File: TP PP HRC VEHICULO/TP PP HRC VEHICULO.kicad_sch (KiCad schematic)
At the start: 56 parts, among them J10 Conn_01x04_Pin, J2 Conn_01x01_Pin, J3 Conn_01x01_Pin, J5vgnd1 Screw_Terminal_01x02, J6 Conn_01x04_Pin, J7 USB_B, J9 Conn_01x04_Pin, K1 Relay_SPDT, K2 Relay_SPDT, SW1 SW_Push, SW2 SW_Push, U1 ESP32-Devkit-V1, U2 LM317L_TO92

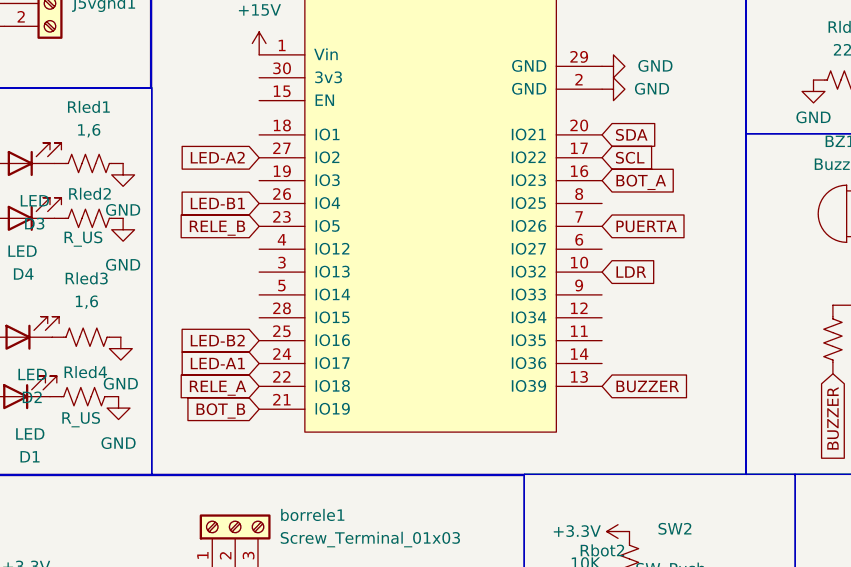
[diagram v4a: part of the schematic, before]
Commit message: terminado
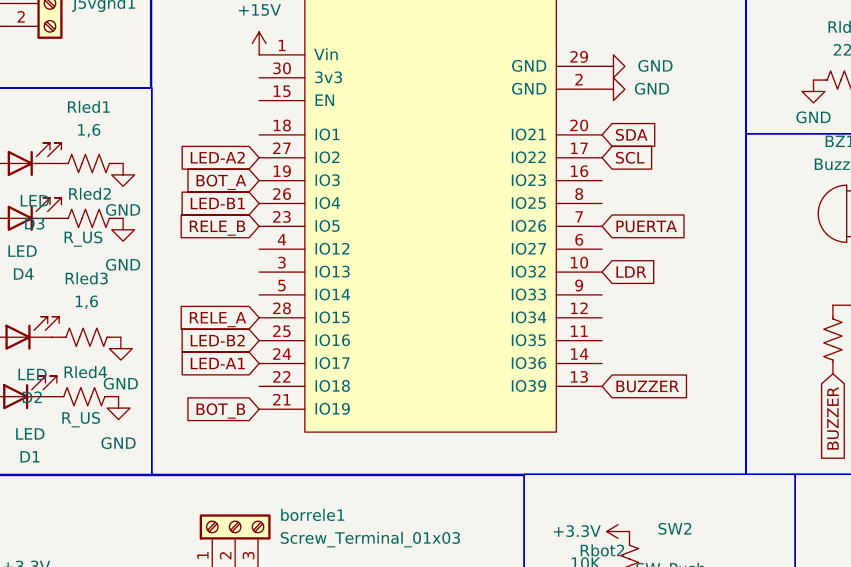
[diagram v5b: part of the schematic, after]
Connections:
- net BOT_A: now also U1.19 (IO3); no longer U1.16 (IO23)
- net RELE_A: now also U1.28 (IO15); no longer U1.22 (IO18)
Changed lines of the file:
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@@
 	(global_label "BOT_A"
 		(shape input)
-		(at 91.694 42.418 0)
-		(fields_autoplaced yes)
-		(effects
-			(font
-				(size 1.27 1.27)
-			)
-			(justify left)
-		)
-		(property "Intersheetrefs" "${INTERSHEET_REFS}"
-			(at 100.3035 42.418 0)
-			(effects
-				(font
-					(size 1.27 1.27)
-				)
-				(justify left)
+		(at 53.594 42.418 180)
+		(fields_autoplaced yes)
+		(effects
+			(font
+				(size 1.27 1.27)
+			)
+			(justify right)
+		)
+		(property "Intersheetrefs" "${INTERSHEET_REFS}"
+			(at 44.9845 42.418 0)
+			(effects
+				(font
+					(size 1.27 1.27)
+				)
+				(justify right)
 				(hide yes)
 			)
@@
 		)
 	)
+	(global_label "LED-A1"
+		(shape input)
+		(at 53.594 62.738 180)
+		(fields_autoplaced yes)
+		(effects
+			(font
+				(size 1.27 1.27)
+			)
+			(justify right)
+		)
+		(property "Intersheetrefs" "${INTERSHEET_REFS}"
+			(at 43.2912 62.738 0)
+			(effects
+				(font
+					(size 1.27 1.27)
+				)
+				(justify right)
+				(hide yes)
+			)
+		)
+	)
+	(global_label "PUERTA"
+		(shape input)
+		(at 91.694 47.498 0)
+		(fields_autoplaced yes)
+		(effects
+			(font
+				(size 1.27 1.27)
+			)
+			(justify left)
+		)
+		(property "Intersheetrefs" "${INTERSHEET_REFS}"
+			(at 101.7549 47.498 0)
+			(effects
+				(font
+					(size 1.27 1.27)
+				)
+				(justify left)
+				(hide yes)
+			)
+		)
+	)
+	(global_label "LDR"
+		(shape input)
+		(at 125.095 31.242 0)
+		(fields_autoplaced yes)
+		(effects
+			(font
+				(size 1.27 1.27)
+			)
+			(justify left)
+		)
+		(property "Intersheetrefs" "${INTERSHEET_REFS}"
+			(at 131.6483 31.242 0)
+			(effects
+				(font
+					(size 1.27 1.27)
+				)
+				(justify left)
+				(hide yes)
+			)
+		)
+	)
+	(global_label "BUZZER"
+		(shape input)
+		(at 117.348 63.881 270)
+		(fields_autoplaced yes)
+		(effects
+			(font
+				(size 1.27 1.27)
+			)
+			(justify right)
+		)
+		(property "Intersheetrefs" "${INTERSHEET_REFS}"
+			(at 117.348 74.3047 90)
+			(effects
+				(font
+					(size 1.27 1.27)
+				)
+				(justify right)
+				(hide yes)
+			)
+		)
+	)
+	(global_label "RELE_B"
+		(shape input)
+		(at 37.338 115.824 270)
+		(fields_autoplaced yes)
+		(effects
+			(font
+				(size 1.27 1.27)
+			)
+			(justify right)
+		)
+		(property "Intersheetrefs" "${INTERSHEET_REFS}"
+			(at 37.338 125.6429 90)
+			(effects
+				(font
+					(size 1.27 1.27)
+				)
+				(justify right)
+				(hide yes)
+			)
+		)
+	)
+	(global_label "SCL"
+		(shape input)
+		(at 169.799 148.59 0)
+		(fields_autoplaced yes)
+		(effects
+			(font
+				(size 1.27 1.27)
+			)
+			(justify left)
+		)
+		(property "Intersheetrefs" "${INTERSHEET_REFS}"
+			(at 176.2918 148.59 0)
+			(effects
+				(font
+					(size 1.27 1.27)
+				)
+				(justify left)
+				(hide yes)
+			)
+		)
+	)
 	(global_label "RELE_A"
 		(shape input)
-		(at 53.594 65.278 180)
-		(fields_autoplaced yes)
-		(effects
-			(font
-				(size 1.27 1.27)
-			)
-			(justify right)
-		)
-		(property "Intersheetrefs" "${INTERSHEET_REFS}"
-			(at 43.9565 65.278 0)
-			(effects
-				(font
-					(size 1.27 1.27)
-				)
-				(justify right)
-				(hide yes)
-			)
-		)
-	)
-	(global_label "LED-A1"
-		(shape input)
-		(at 53.594 62.738 180)
-		(fields_autoplaced yes)
-		(effects
-			(font
-				(size 1.27 1.27)
-			)
-			(justify right)
-		)
-		(property "Intersheetrefs" "${INTERSHEET_REFS}"
-			(at 43.2912 62.738 0)
-			(effects
-				(font
-					(size 1.27 1.27)
-				)
-				(justify right)
-				(hide yes)
-			)
-		)
-	)
-	(global_label "PUERTA"
-		(shape input)
-		(at 91.694 47.498 0)
-		(fields_autoplaced yes)
-		(effects
-			(font
-				(size 1.27 1.27)
-			)
-			(justify left)
-		)
-		(property "Intersheetrefs" "${INTERSHEET_REFS}"
-			(at 101.7549 47.498 0)
-			(effects
-				(font
-					(size 1.27 1.27)
-				)
-				(justify left)
-				(hide yes)
-			)
-		)
-	)
-	(global_label "LDR"
-		(shape input)
-		(at 125.095 31.242 0)
-		(fields_autoplaced yes)
-		(effects
-			(font
-				(size 1.27 1.27)
-			)
-			(justify left)
-		)
-		(property "Intersheetrefs" "${INTERSHEET_REFS}"
-			(at 131.6483 31.242 0)
-			(effects
-				(font
-					(size 1.27 1.27)
-				)
-				(justify left)
-				(hide yes)
-			)
-		)
-	)
-	(global_label "BUZZER"
-		(shape input)
-		(at 117.348 63.881 270)
-		(fields_autoplaced yes)
-		(effects
-			(font
-				(size 1.27 1.27)
-			)
-			(justify right)
-		)
-		(property "Intersheetrefs" "${INTERSHEET_REFS}"
-			(at 117.348 74.3047 90)
-			(effects
-				(font
-					(size 1.27 1.27)
-				)
-				(justify right)
-				(hide yes)
-			)
-		)
-	)
-	(global_label "RELE_B"
-		(shape input)
-		(at 37.338 115.824 270)
-		(fields_autoplaced yes)
-		(effects
-			(font
-				(size 1.27 1.27)
-			)
-			(justify right)
-		)
-		(property "Intersheetrefs" "${INTERSHEET_REFS}"
-			(at 37.338 125.6429 90)
-			(effects
-				(font
-					(size 1.27 1.27)
-				)
-				(justify right)
-				(hide yes)
-			)
-		)
-	)
-	(global_label "SCL"
-		(shape input)
-		(at 169.799 148.59 0)
-		(fields_autoplaced yes)
-		(effects
-			(font
-				(size 1.27 1.27)
-			)
-			(justify left)
-		)
-		(property "Intersheetrefs" "${INTERSHEET_REFS}"
-			(at 176.2918 148.59 0)
-			(effects
-				(font
-					(size 1.27 1.27)
-				)
-				(justify left)
-				(hide yes)
-			)
+		(at 53.594 57.658 180)
+		(fields_autoplaced yes)
+		(effects
+			(font
+				(size 1.27 1.27)
+			)
+			(justify right)
+		)
+		(property "Intersheetrefs" "${INTERSHEET_REFS}"
+			(at 43.9565 57.658 0)
+			(effects
+				(font
+					(size 1.27 1.27)
+				)
+				(justify right)
+				(hide yes)
+			)

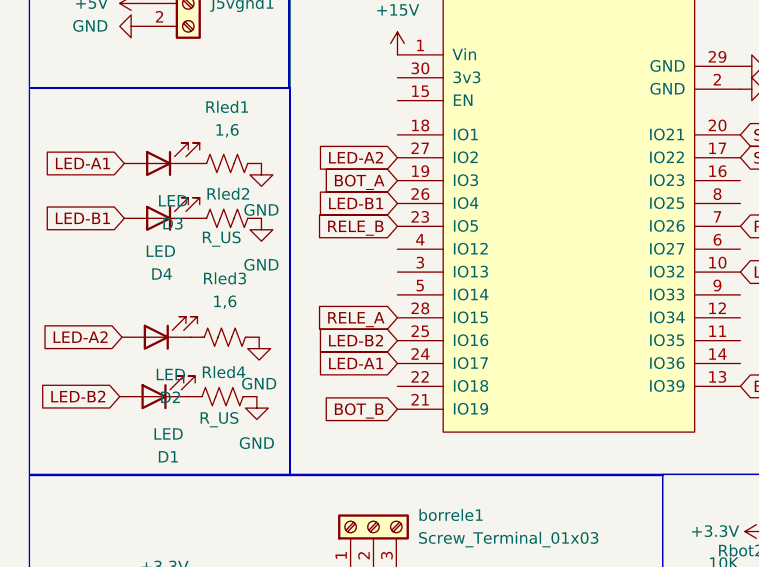
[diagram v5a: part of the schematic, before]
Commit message: t
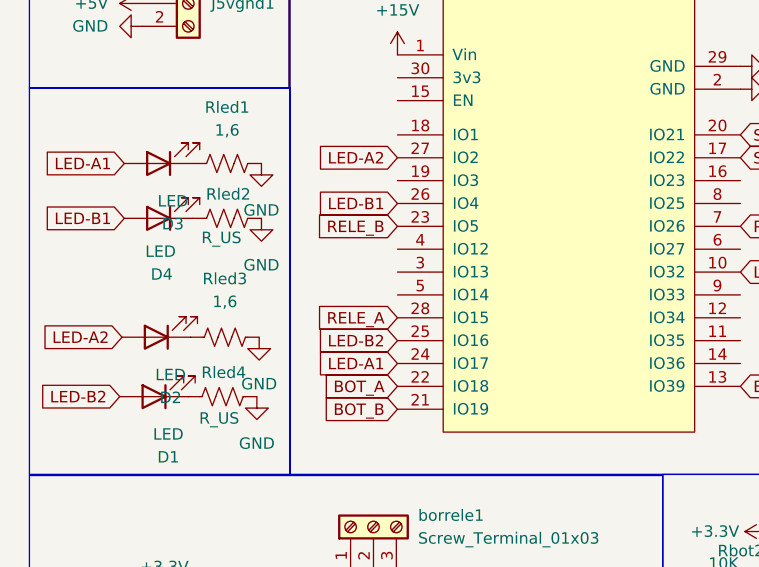
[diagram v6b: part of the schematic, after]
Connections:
- net BOT_A: now also U1.22 (IO18); no longer U1.19 (IO3)
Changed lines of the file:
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@@
+		)
+	)
+	(global_label "BOT_A"
+		(shape input)
+		(at 53.594 65.278 180)
+		(fields_autoplaced yes)
+		(effects
+			(font
+				(size 1.27 1.27)
+			)
+			(justify right)
+		)
+		(property "Intersheetrefs" "${INTERSHEET_REFS}"
+			(at 44.9845 65.278 0)
+			(effects
+				(font
+					(size 1.27 1.27)
+				)
+				(justify right)
+				(hide yes)
+			)
 		)
 	)
@@
 			(effects
 				(font
-					(size 1.27 1.27)
-				)
-				(justify right)
-				(hide yes)
-			)
-		)
-	)
-	(global_label "BOT_A"
-		(shape input)
-		(at 53.594 42.418 180)
-		(fields_autoplaced yes)
-		(effects
-			(font
-				(size 1.27 1.27)
-			)
-			(justify right)
-		)
-		(property "Intersheetrefs" "${INTERSHEET_REFS}"
-			(at 44.9845 42.418 0)
-			(effects
-				(font
